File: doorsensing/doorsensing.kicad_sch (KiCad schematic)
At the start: 2 parts, among them U1 ADS1115IDGSR, U2 OPA333xxD

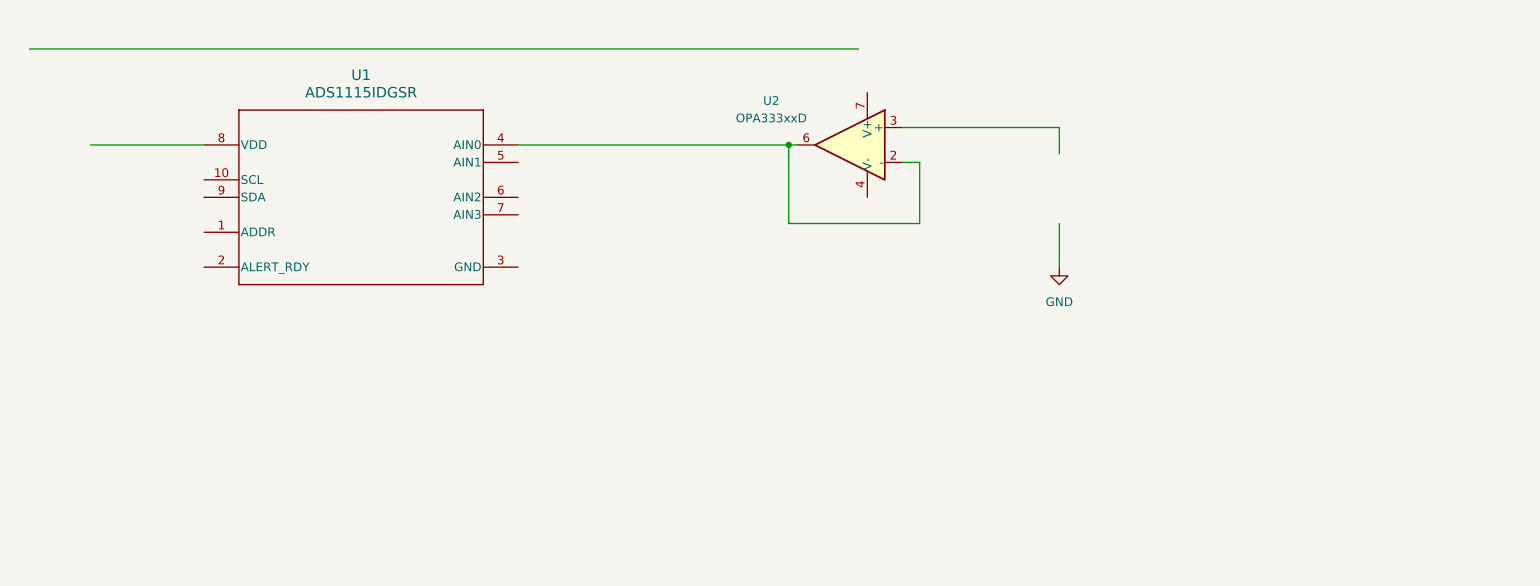
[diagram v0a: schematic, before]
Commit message: continued working schematic
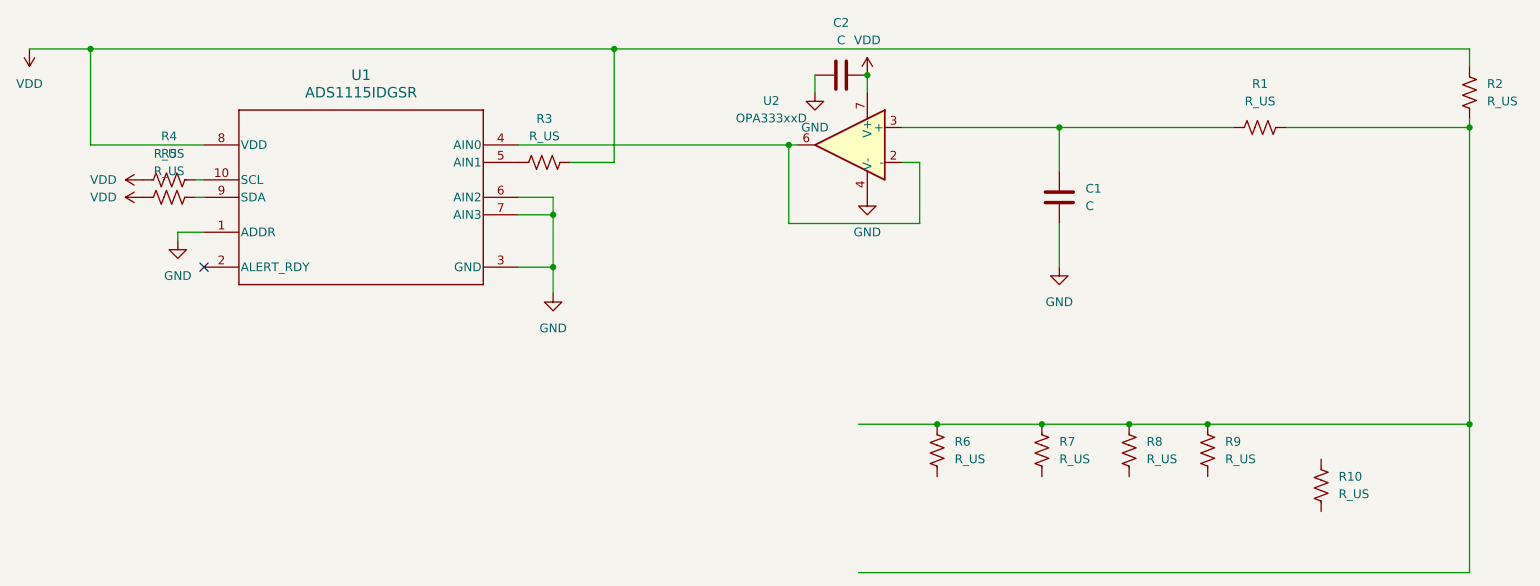
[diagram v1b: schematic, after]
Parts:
- added C1, C2: C, symbol Device:C
- added R1, R10, R2, R3, R4, R5, R6, R7, R8, R9: R_US, symbol Device:R_US
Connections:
- net GND: now also U1.1 (ADDR), U1.3 (GND), U1.6 (AIN2), U1.7 (AIN3), U2.4 (V-), C1.2, C2.1
- net at U1.10 (SCL): now also R4.2
- net at U1.5 (AIN1): now also R3.1
- net VDD: now reaches U1.8 (VDD)
- net VDD: now also U2.7 (V+), C2.2, R2.1, R3.2, R4.1, R5.1
- net at U1.9 (SDA): now also R5.2
- net at U2.3 (+): now also C1.1, R1.2
- new net: R1.1, R2.2, R6.1, R7.1, R8.1, R9.1
- no-connect marks 0 -> 1
